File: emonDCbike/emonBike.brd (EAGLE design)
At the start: 99.1 x 76.5 mm, 85 parts, among them Q1 16Mhz XT49M-2016M, U1_TQFP ATMEGA328P

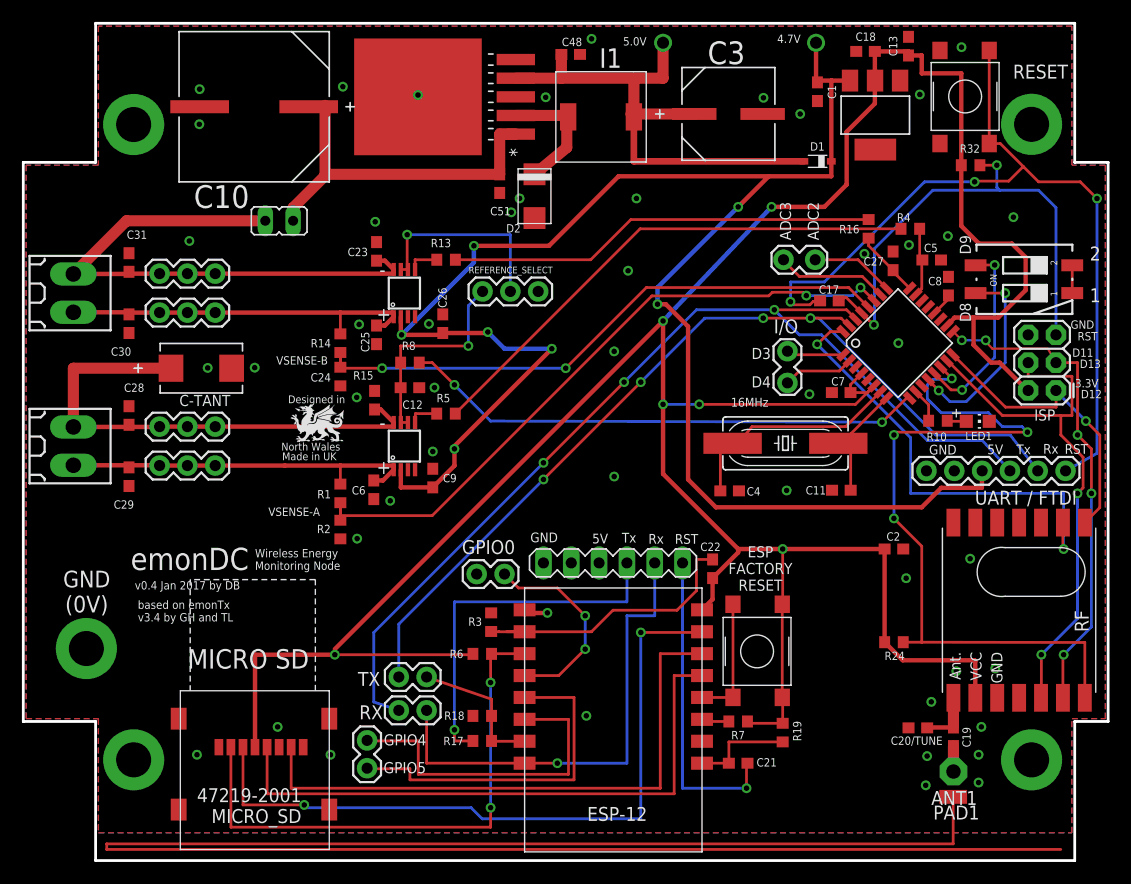
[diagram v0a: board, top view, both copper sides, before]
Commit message: emonDCbike design first draft
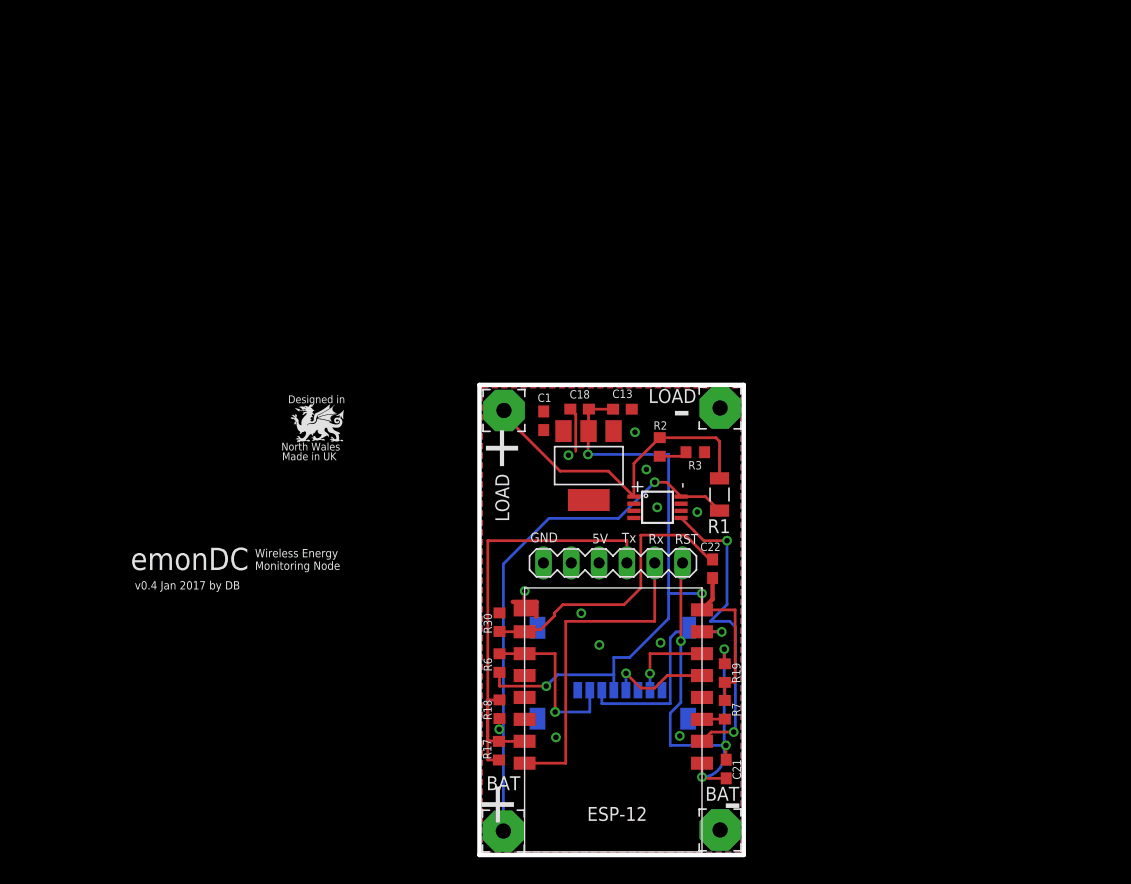
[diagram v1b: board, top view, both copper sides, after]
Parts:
- removed 5V_REG: TL2575HV, TL2575HV:TO-263
- removed ANA, I/O: 2212S-02SG-85, SparkFun-Connectors:1X02_LOCK
- removed ANT1: (no value), discrete:PAD-01
- removed C-TANT: 10uF 63V, 2917 footprint capacitor:2917
- removed C10: 100uF 80V, Panasonic-EEE-EEV-EEF-ECQ:CAPAE1350X1400N
- removed C11, C19, C4: 22pF, rcl:C0603
- removed C12: 220nF, rcl:C0603
- removed C17, C2, C27, C48, C5, C51, C7, C8: 100nF, rcl:C0603
- removed C20/TUNE: tune, rcl:C0603
- removed C23, C24, C25, C26, C28, C29, C30, C31, C6, C9: 0.1uF 100V, rcl:C0603
- removed C3: 470uF, Panasonic-EEEFK_EEEFP:CAPAE830X1050N
- removed D1: BAT60J, diode:SOD323_ST
- removed D2: MBRA130LT3G, CASE 403D Diode:DO-214
- removed FTDI/UART: 2211S-06G, SparkFun:FTDI_BASIC
- removed GPIO-4/5, GPIO0, RX, TX: (no value), SparkFun:1X02
- removed I1: 330uH, SRR0603-331KL:SRR0603-331KL
- removed ISP: M20-9980346, SparkFun:2X3
- removed J1, J2, J3, J4: (no value), SparkFun-Connectors:1X03
- removed JP3: 2211S-02G, jumper:JP1
- removed LED1: Red 1.85V, adafruit:CHIP-LED0805
- removed MC1, MC32882: MC32882, multicomp tact switch:SWITCH_TACT_MULTICOMP
- removed Q1: 16Mhz XT49M-2016M, adafruit:HC49UP
- removed R10, R13, R5: 1K, rcl:R0603
- removed R14: 100K 60V, rcl:R0603
- removed R15: 5.9K, rcl:R0603
- removed R16, R4: 9K1, rcl:R0603
- removed R24: 120K, rcl:R0603
- removed R32: 10K, rcl:R0603
- removed R8: 3.9K, rcl:R0603
- removed REFERENCE_SELECT: 2212S-02SG-85, SparkFun-Connectors:1X03
- removed RF: RFM12B, JeeParts:RFM12B
- removed S3: A6S-2104-PH, OpenEnergyMonitor:DIP_SWITCH_SMT
- removed SHUNTMON-B: LMP8481, lmp8481b:S-PDSO-G08
- removed T1, T2: (no value), con-weidmueller-sl35:180-2
- removed U1_TQFP: ATMEGA328P, SparkFun-DigitalIC:TQFP32-08
- added PAD2, PAD3, PAD4: (no value), wirepad:3,81/1,4
- added R30: 10k, rcl:R0603
- PAD1: device wirepad:SMD1,27-2,54 -> wirepad:3,81/1,4
- R1: value 100K 60V -> 0.022 OHM; device rcl:R0603 -> Panasonic-ERJ3_ERJ8_ERJA_ERJB:RESC3216X71N
- R2: value 5.9K -> 100K 60V
- R3: value 10k -> 5.9K
- moved C13 42.2 mm to (55.0, 43.0), turned to 0 degrees
- moved C18 41.8 mm to (51.1, 43.0)
- moved 3.3V_REG 41.3 mm to (51.9, 37.8)
- moved PAD1 41.2 mm to (44.1, 4.47), turned to 0 degrees
- moved C1 39.1 mm to (47.8, 41.9), turned to 90 degrees
- moved R1 34.6 mm to (63.8, 35.2)
- moved U$1 32.8 mm to (61.0, 14.7), flipped to the bottom, turned to 0 degrees
- moved SHUNTMON-A 30.3 mm to (58.2, 34.0), turned to 270 degrees
- moved R2 30.1 mm to (58.4, 39.5)
- moved R3 24.3 mm to (61.6, 39.1), turned to 180 degrees
- moved R19 7.58 mm to (64.3, 18.9), turned to 270 degrees
- moved R6 1.78 mm to (43.7, 19.8), turned to 270 degrees
- moved R17 1.76 mm to (43.7, 11.8), turned to 90 degrees
- moved R18 1.69 mm to (43.7, 15.6), turned to 270 degrees
- moved R7 1.62 mm to (64.3, 15.5), turned to 90 degrees
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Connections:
- removed net ADC2: ANA.1, U1_TQFP.25
- removed net ADC3: ANA.2, U1_TQFP.26
- removed net ADCSHUNT-A: R13.2, R16.2
- removed net ADCSHUNT-B: R4.2, R5.2
- removed net ADCVSENSE-B: R1.1, R2.2, U1_TQFP.27
- removed net AGND: U1_TQFP.21
- removed net D0/RX: FTDI/UART.TXO, RX.2, U1_TQFP.30
- removed net D1/TX: FTDI/UART.RXI, TX.2, U1_TQFP.31
- removed net D10: R24.1, RF.SEL, U1_TQFP.14
- removed net D11/MOSI: ISP.4, RF.SDI, U1_TQFP.15
- removed net D12/MISO: ISP.1, RF.SDO, U1_TQFP.16
- removed net D13/SCK: ISP.3, RF.SCK, U1_TQFP.17
- removed net D2: RF.IRQ, U1_TQFP.32
- removed net D3: I/O.1, U1_TQFP.1
- removed net D4: I/O.2, U1_TQFP.2
- removed net D5/PWM0: R8.2, U1_TQFP.9
- removed net D6: R10.2, U1_TQFP.10
- removed net D7: U1_TQFP.11
- removed net D8: S3.4, U1_TQFP.12
- removed net D9: S3.3, U1_TQFP.13
- removed net DIG1: C19.1, C20/TUNE.1, RF.ANT
- removed net IND: 5V_REG.2, D2.P$1, I1.P$1
- removed net INPUT-POS-B: C29.1, C6.1, J3.1, J3.2, J3.3, R1.2, SHUNTMON-B.1, T2.2
- removed net LOAD-NEG-B: C-TANT.1, C24.2, C28.1, J4.1, J4.2, J4.3, SHUNTMON-B.8, T2.1
- removed net N$1: C4.1, Q1.2, U1_TQFP.7
- removed net N$2: C5.2, R4.1, U1_TQFP.23
- removed net N$20: C8.1, U1_TQFP.20
- removed net N$27: C27.2, R16.1, U1_TQFP.24
- removed net N$28: REFERENCE_SELECT.2, SHUNTMON-A.6, SHUNTMON-A.7
- removed net N$3: ANT1.1, C19.2
- removed net N$4: R13.1, SHUNTMON-A.5
- removed net N$41: LED1.A, R10.1
- removed net N$5: PAD1.1
- removed net N$6: R5.1, SHUNTMON-B.5
- removed net N$9: C11.1, Q1.1, U1_TQFP.8
- removed net POWERIN: 5V_REG.1, C10.1, C51.1, JP3.1
- removed net REFINPUT: C12.1, R8.1, REFERENCE_SELECT.1, SHUNTMON-B.6, SHUNTMON-B.7
- removed net RES: C17.1, FTDI/UART.DTR, MC32882.P$1, MC32882.P$2
- removed net RESET: C17.2, ISP.5, R32.1, U1_TQFP.29
- net 3.3V: no longer C2.1, C7.1, ISP.2, MC1.P$3, MC1.P$4, R24.2, R32.2, RF.VDD, U1_TQFP.18, U1_TQFP.4, U1_TQFP.6
- net 4.7V: no longer 3.3V_REG.3, C1.1, C26.1, C9.1, D1.C, FTDI/UART.VCC, SHUNTMON-B.2
- net 5.0V: now also 3.3V_REG.3, C1.1; no longer 5V_REG.4, C3.1, C48.1, D1.A, I1.P$2
- net ADC: now also SHUNTMON-A.5
- net ADCVSENSE-A: now also R2.1, R3.2; no longer R14.1, R15.2, U1_TQFP.28
- net ESPRX: no longer TX.1
- net ESPTX: no longer RX.1
- net GND: now also PAD3.1, PAD4.1, R30.1, SHUNTMON-A.6, SHUNTMON-A.7; no longer 5V_REG.3, 5V_REG.5, 5V_REG.6, C-TANT.2, C10.2, C11.2, C12.2, C2.2, C20/TUNE.2, C23.1, C24.1, C25.2, C26.2, C27.1, C28.2, C29.2, C3.2, C30.2, C31.2, C4.2, C48.2, C5.1, C51.2, C6.2, C7.2, C8.2, C9.2, D2.P$2, FTDI/UART.GND, GPIO0.1, ISP.6, LED1.C, MC32882.P$3, MC32882.P$4, R15.1, R2.1, REFERENCE_SELECT.3, RF.GND, RF.P$12, S3.1, S3.2, SHUNTMON-B.4, U1_TQFP.3, U1_TQFP.5
- net GPIO0: no longer GPIO0.2
- net GPIO15: now also R30.2; no longer R3.2
- net GPIO16: no longer MC1.P$1, MC1.P$2
- net GPIO4: no longer GPIO-4/5.1
- net GPIO5: no longer GPIO-4/5.2
- net INPUT-POS-A: now also PAD2.1, R1.2, R2.2; no longer C25.1, C30.1, J2.1, J2.2, J2.3, R14.2, T1.2
- net LOAD-NEG-A: now also PAD1.1, R1.1; no longer C23.2, C31.1, J1.1, J1.2, J1.3, JP3.2, T1.1
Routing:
- net 3.3V: track 267.5 -> 70.4 mm, vias 6 -> 3
- net N$31: track 168.7 -> 0.00 mm
- net 4.7V: track 163.5 -> 0.00 mm, vias 8 -> 0
- net D0/RX: track 93.0 -> 0.00 mm, vias 3 -> 0
- net D1/TX: track 84.6 -> 0.00 mm, vias 4 -> 0
- net RES: track 77.6 -> 0.00 mm, vias 3 -> 0
- net D10: track 69.7 -> 0.00 mm, vias 4 -> 0
- net ADCVSENSE-B: track 60.9 -> 0.00 mm, vias 2 -> 0
- net ADCVSENSE-A: track 54.7 -> 2.55 mm, vias 2 -> 0
- net D11/MOSI: track 50.6 -> 0.00 mm, vias 2 -> 0
- net LOAD-NEG-B: track 48.4 -> 0.00 mm
- net 5.0V: track 48.1 -> 0.00 mm, vias 1 -> 0
- net D5/PWM0: track 48.0 -> 0.00 mm, vias 2 -> 0
- net ADCSHUNT-B: track 47.7 -> 0.00 mm
- net RESET: track 46.3 -> 0.00 mm, vias 2 -> 0
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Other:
- board size 99.1 x 76.5 mm -> 24.1 x 42.9 mm
- board text added: "+"
- board text added: "-"
- board text added: "BAT"
- board text added: "LOAD"
- board text removed: "16MHz"
- board text removed: "2 1"
- board text removed: "3.3V"
- board text removed: "4.7V"
- board text removed: "5.0V"
- board text removed: "A"
- board text removed: "ADC2"
- board text removed: "ADC3"
- board text removed: "B"
- board text removed: "D11"
- board text removed: "D12"
- board text removed: "D13"
- board text removed: "D2"
- board text removed: "D3"
- board text removed: "D4"
- board text removed: "D8"
- board text removed: "D9"
- board text removed: "Designed in North Wales UK by Megni"
- board text removed: "ESP FACTORY RESET"
- board text removed: "GND (0V)"
- board text removed: "GPIO4"
- board text removed: "GPIO5"
- board text removed: "I1"
- board text removed: "MICRO SD"
- board text removed: "Node:"
- board text removed: "OpenEnergyMonitor.org"
- board text removed: "RESET"
- board text removed: "UART / FTDI"
- board text removed: "VSENSE-A"
- board text removed: "VSENSE-B"
- board text removed: "based on emonTx v3.4 by GH and TL"
